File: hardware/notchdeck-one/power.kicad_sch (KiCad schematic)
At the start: 21 parts, among them J1 USB-C, J2 BAT 1S, Q1 AO3401A, U2 AP2112K-3.3, U3 MCP73831-2-OT, U4 MAX17048, U7 USBLC6-2SC6, U8 74LVC1G125

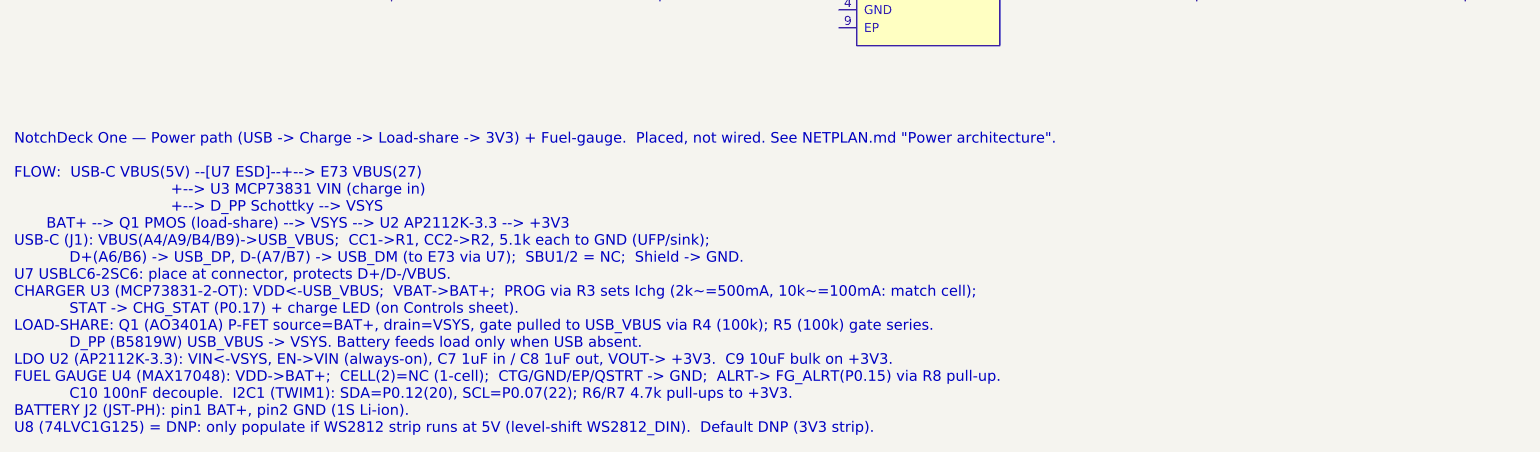
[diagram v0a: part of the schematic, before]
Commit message: Add schematic wiring notes support
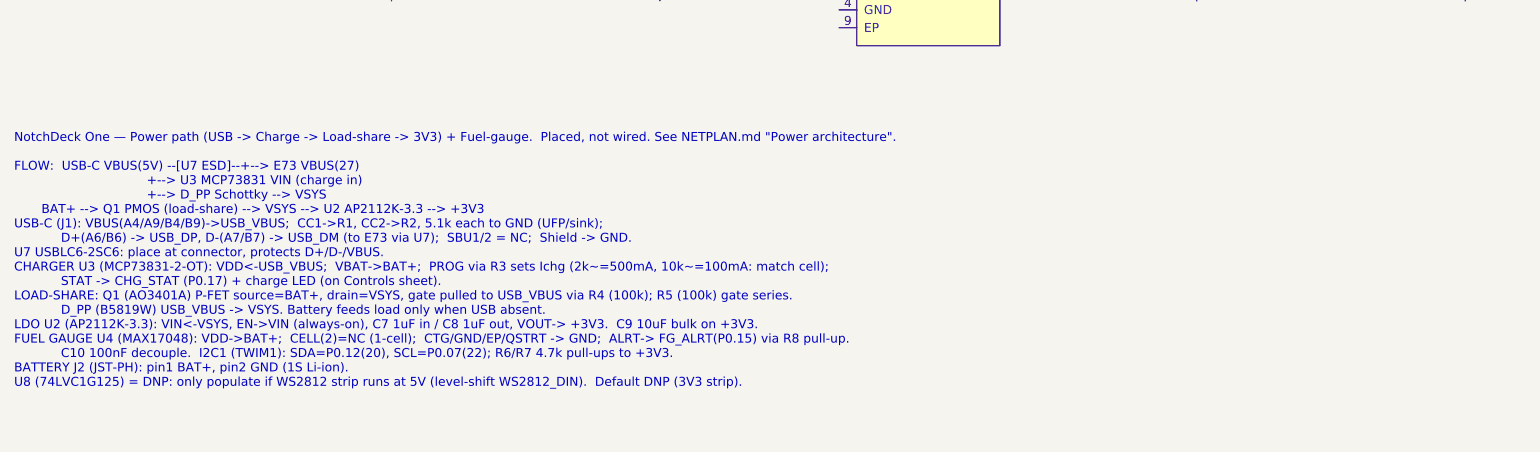
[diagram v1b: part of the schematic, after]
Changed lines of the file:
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@@
 		(instances
 			(project "notchdeck-one"
-				(path "/9b1c0f7a-1d2e-4a3b-8c5d-0e6f7a8b9c01/7d2dd40e-5097-4a0f-9306-a516a342b95f"
+				(path "/9b1c0f7a-1d2e-4a3b-8c5d-0e6f7a8b9c01/2c77e6d8-3afb-4a5f-bda1-2cf5540b755c"
 					(reference "J1")
 					(unit 1)
@@
 		(instances
 			(project "notchdeck-one"
-				(path "/9b1c0f7a-1d2e-4a3b-8c5d-0e6f7a8b9c01/7d2dd40e-5097-4a0f-9306-a516a342b95f"
+				(path "/9b1c0f7a-1d2e-4a3b-8c5d-0e6f7a8b9c01/2c77e6d8-3afb-4a5f-bda1-2cf5540b755c"
 					(reference "U7")
 					(unit 1)
@@
 		(instances
 			(project "notchdeck-one"
-				(path "/9b1c0f7a-1d2e-4a3b-8c5d-0e6f7a8b9c01/7d2dd40e-5097-4a0f-9306-a516a342b95f"
+				(path "/9b1c0f7a-1d2e-4a3b-8c5d-0e6f7a8b9c01/2c77e6d8-3afb-4a5f-bda1-2cf5540b755c"
 					(reference "R1")
 					(unit 1)
@@
 		(instances
 			(project "notchdeck-one"
-				(path "/9b1c0f7a-1d2e-4a3b-8c5d-0e6f7a8b9c01/7d2dd40e-5097-4a0f-9306-a516a342b95f"
+				(path "/9b1c0f7a-1d2e-4a3b-8c5d-0e6f7a8b9c01/2c77e6d8-3afb-4a5f-bda1-2cf5540b755c"
 					(reference "R2")
 					(unit 1)
@@
 		(instances
 			(project "notchdeck-one"
-				(path "/9b1c0f7a-1d2e-4a3b-8c5d-0e6f7a8b9c01/7d2dd40e-5097-4a0f-9306-a516a342b95f"
+				(path "/9b1c0f7a-1d2e-4a3b-8c5d-0e6f7a8b9c01/2c77e6d8-3afb-4a5f-bda1-2cf5540b755c"
 					(reference "U3")
 					(unit 1)
@@
 		(instances
 			(project "notchdeck-one"
-				(path "/9b1c0f7a-1d2e-4a3b-8c5d-0e6f7a8b9c01/7d2dd40e-5097-4a0f-9306-a516a342b95f"
+				(path "/9b1c0f7a-1d2e-4a3b-8c5d-0e6f7a8b9c01/2c77e6d8-3afb-4a5f-bda1-2cf5540b755c"
 					(reference "R3")
 					(unit 1)
@@
 		(instances
 			(project "notchdeck-one"
-				(path "/9b1c0f7a-1d2e-4a3b-8c5d-0e6f7a8b9c01/7d2dd40e-5097-4a0f-9306-a516a342b95f"
+				(path "/9b1c0f7a-1d2e-4a3b-8c5d-0e6f7a8b9c01/2c77e6d8-3afb-4a5f-bda1-2cf5540b755c"
 					(reference "U2")
 					(unit 1)
@@
 		(instances
 			(project "notchdeck-one"
-				(path "/9b1c0f7a-1d2e-4a3b-8c5d-0e6f7a8b9c01/7d2dd40e-5097-4a0f-9306-a516a342b95f"
+				(path "/9b1c0f7a-1d2e-4a3b-8c5d-0e6f7a8b9c01/2c77e6d8-3afb-4a5f-bda1-2cf5540b755c"
 					(reference "C7")
 					(unit 1)
@@
 		(instances
 			(project "notchdeck-one"
-				(path "/9b1c0f7a-1d2e-4a3b-8c5d-0e6f7a8b9c01/7d2dd40e-5097-4a0f-9306-a516a342b95f"
+				(path "/9b1c0f7a-1d2e-4a3b-8c5d-0e6f7a8b9c01/2c77e6d8-3afb-4a5f-bda1-2cf5540b755c"
 					(reference "C8")
 					(unit 1)
@@
 		(instances
 			(project "notchdeck-one"
-				(path "/9b1c0f7a-1d2e-4a3b-8c5d-0e6f7a8b9c01/7d2dd40e-5097-4a0f-9306-a516a342b95f"
+				(path "/9b1c0f7a-1d2e-4a3b-8c5d-0e6f7a8b9c01/2c77e6d8-3afb-4a5f-bda1-2cf5540b755c"
 					(reference "C9")
 					(unit 1)
@@
 		(instances
 			(project "notchdeck-one"
-				(path "/9b1c0f7a-1d2e-4a3b-8c5d-0e6f7a8b9c01/7d2dd40e-5097-4a0f-9306-a516a342b95f"
+				(path "/9b1c0f7a-1d2e-4a3b-8c5d-0e6f7a8b9c01/2c77e6d8-3afb-4a5f-bda1-2cf5540b755c"
 					(reference "Q1")
 					(unit 1)
@@
 		(instances
 			(project "notchdeck-one"
-				(path "/9b1c0f7a-1d2e-4a3b-8c5d-0e6f7a8b9c01/7d2dd40e-5097-4a0f-9306-a516a342b95f"
+				(path "/9b1c0f7a-1d2e-4a3b-8c5d-0e6f7a8b9c01/2c77e6d8-3afb-4a5f-bda1-2cf5540b755c"
 					(reference "D_PP")
 					(unit 1)
@@
 		(instances
 			(project "notchdeck-one"
-				(path "/9b1c0f7a-1d2e-4a3b-8c5d-0e6f7a8b9c01/7d2dd40e-5097-4a0f-9306-a516a342b95f"
+				(path "/9b1c0f7a-1d2e-4a3b-8c5d-0e6f7a8b9c01/2c77e6d8-3afb-4a5f-bda1-2cf5540b755c"
 					(reference "R4")
 					(unit 1)
@@
 		(instances
 			(project "notchdeck-one"
-				(path "/9b1c0f7a-1d2e-4a3b-8c5d-0e6f7a8b9c01/7d2dd40e-5097-4a0f-9306-a516a342b95f"
+				(path "/9b1c0f7a-1d2e-4a3b-8c5d-0e6f7a8b9c01/2c77e6d8-3afb-4a5f-bda1-2cf5540b755c"
 					(reference "R5")
 					(unit 1)
@@
 		(instances
 			(project "notchdeck-one"
-				(path "/9b1c0f7a-1d2e-4a3b-8c5d-0e6f7a8b9c01/7d2dd40e-5097-4a0f-9306-a516a342b95f"
+				(path "/9b1c0f7a-1d2e-4a3b-8c5d-0e6f7a8b9c01/2c77e6d8-3afb-4a5f-bda1-2cf5540b755c"
 					(reference "U4")
 					(unit 1)
@@
 		(instances
 			(project "notchdeck-one"
-				(path "/9b1c0f7a-1d2e-4a3b-8c5d-0e6f7a8b9c01/7d2dd40e-5097-4a0f-9306-a516a342b95f"
+				(path "/9b1c0f7a-1d2e-4a3b-8c5d-0e6f7a8b9c01/2c77e6d8-3afb-4a5f-bda1-2cf5540b755c"
 					(reference "C10")
 					(unit 1)
@@
 		(instances
 			(project "notchdeck-one"
-				(path "/9b1c0f7a-1d2e-4a3b-8c5d-0e6f7a8b9c01/7d2dd40e-5097-4a0f-9306-a516a342b95f"
+				(path "/9b1c0f7a-1d2e-4a3b-8c5d-0e6f7a8b9c01/2c77e6d8-3afb-4a5f-bda1-2cf5540b755c"
 					(reference "R6")
 					(unit 1)
@@
 		(instances
 			(project "notchdeck-one"
-				(path "/9b1c0f7a-1d2e-4a3b-8c5d-0e6f7a8b9c01/7d2dd40e-5097-4a0f-9306-a516a342b95f"
+				(path "/9b1c0f7a-1d2e-4a3b-8c5d-0e6f7a8b9c01/2c77e6d8-3afb-4a5f-bda1-2cf5540b755c"
 					(reference "R7")
 					(unit 1)
@@
 		(instances
 			(project "notchdeck-one"
-				(path "/9b1c0f7a-1d2e-4a3b-8c5d-0e6f7a8b9c01/7d2dd40e-5097-4a0f-9306-a516a342b95f"
+				(path "/9b1c0f7a-1d2e-4a3b-8c5d-0e6f7a8b9c01/2c77e6d8-3afb-4a5f-bda1-2cf5540b755c"
 					(reference "R8")
 					(unit 1)
@@
 		(instances
 			(project "notchdeck-one"
-				(path "/9b1c0f7a-1d2e-4a3b-8c5d-0e6f7a8b9c01/7d2dd40e-5097-4a0f-9306-a516a342b95f"
+				(path "/9b1c0f7a-1d2e-4a3b-8c5d-0e6f7a8b9c01/2c77e6d8-3afb-4a5f-bda1-2cf5540b755c"
 					(reference "J2")
 					(unit 1)
@@
 		(instances
 			(project "notchdeck-one"
-				(path "/9b1c0f7a-1d2e-4a3b-8c5d-0e6f7a8b9c01/7d2dd40e-5097-4a0f-9306-a516a342b95f"
+				(path "/9b1c0f7a-1d2e-4a3b-8c5d-0e6f7a8b9c01/2c77e6d8-3afb-4a5f-bda1-2cf5540b755c"
 					(reference "U8")
 					(unit 1)
@@
 		(exclude_from_sim no)
 		(at 15.00 175.00 0)
-		(effects (font (size 1.5 1.5)) (justify left top))
+		(effects (font (face "Courier New") (size 1.27 1.27)) (justify left top))
 	)
 	(sheet_instances
